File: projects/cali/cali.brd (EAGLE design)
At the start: 100 x 80 mm, 25 parts, among them Q3 IRF540, T1 BC547, T2 BC547, T3 BC547

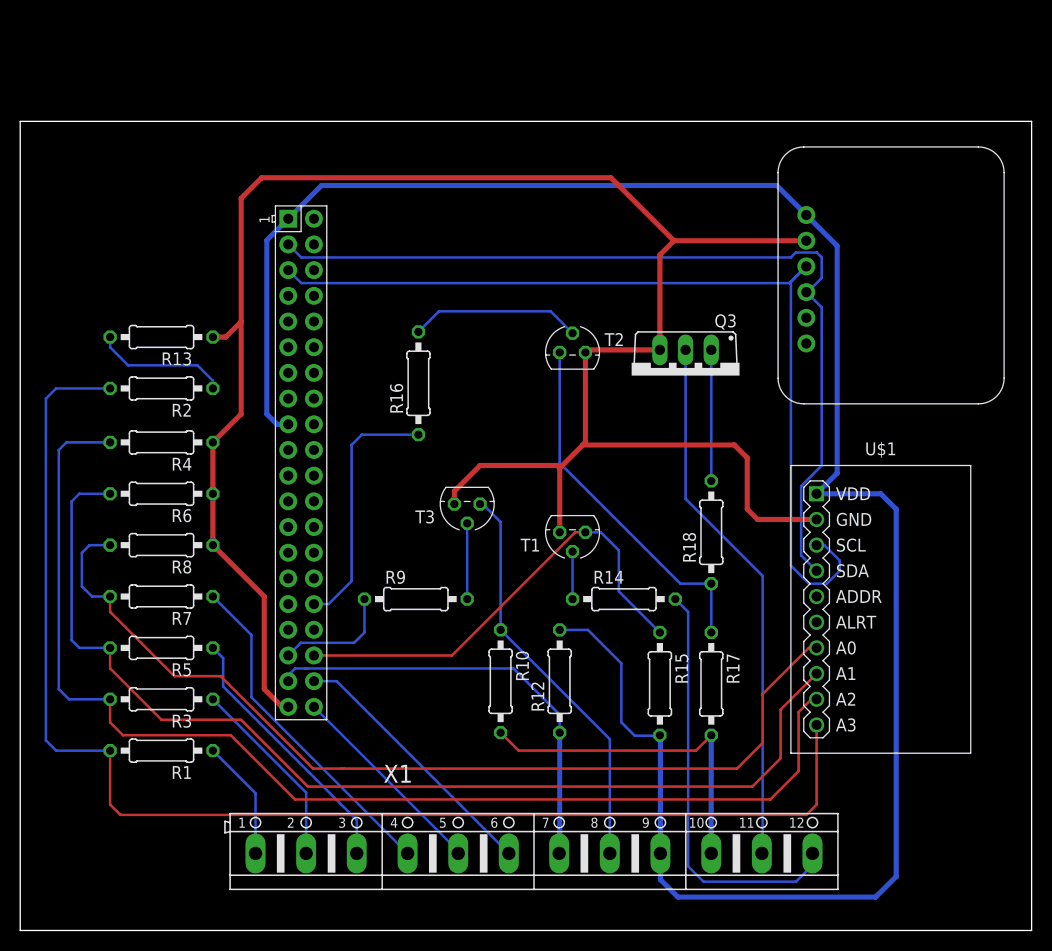
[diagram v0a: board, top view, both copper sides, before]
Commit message: Board v1.0
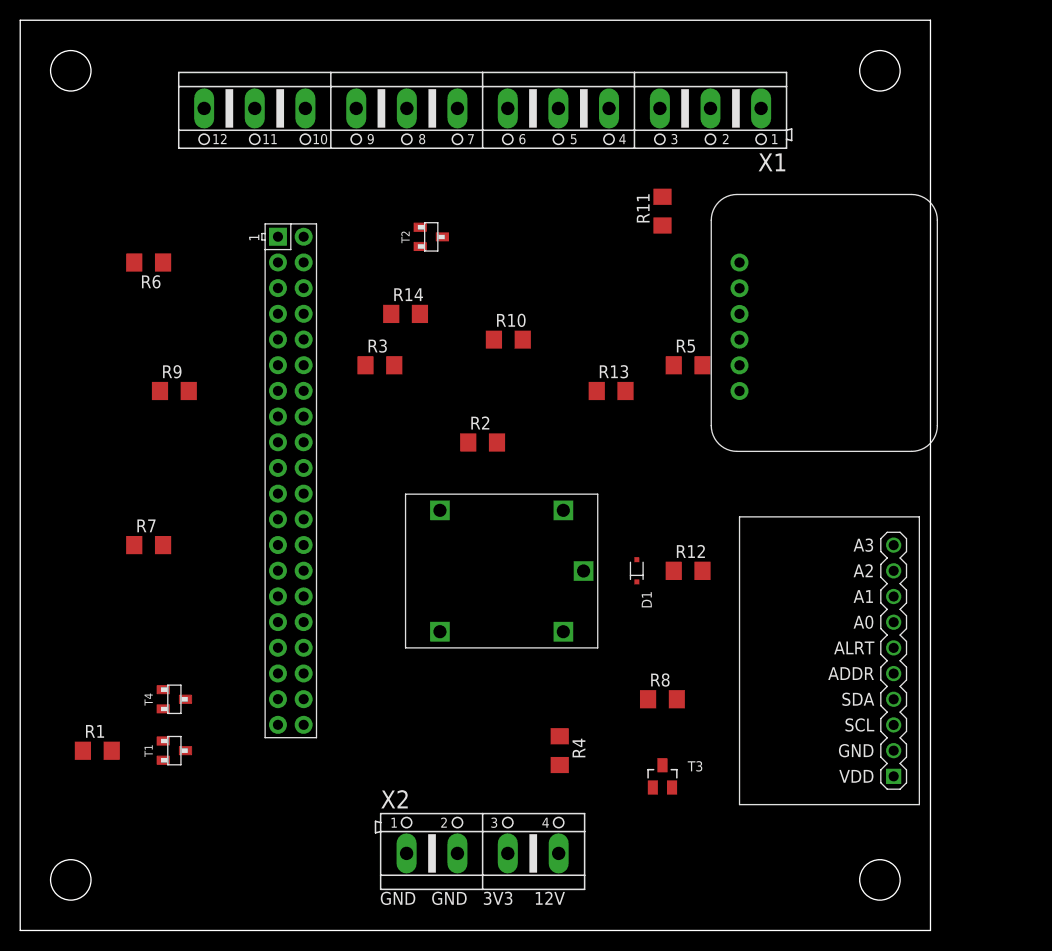
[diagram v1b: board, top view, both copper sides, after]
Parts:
- removed Q3: IRF540, transistor-power:TO220BV
- removed R15, R17: 10k, rcl:0207/10
- removed R16: 1k, rcl:0207/10
- removed R18: 10, rcl:0207/10
- added D1: BAS316, nxp_60:SOD323(F)
- added R11: 10k, rcl:R1206
- added T4: IRLML2502, we-transistor:SOT23
- added U$4: FINDER-36.11, relay2:FINDER-36.11
- added X2: (no value), con-ptr500:AK500/4
- R1: value 0 -> 100; device rcl:0207/10 -> rcl:R1206
- R10: value 10k -> 1k; device rcl:0207/10 -> rcl:R1206
- R12: value 4k7 -> 1k; device rcl:0207/10 -> rcl:R1206
- R13: value 1k -> 0; device rcl:0207/10 -> rcl:R1206
- R14: value 10k -> 2k; device rcl:0207/10 -> rcl:R1206
- R2, R6: value 1k -> 100; device rcl:0207/10 -> rcl:R1206
- R3, R4, R5, R7, R8: device rcl:0207/10 -> rcl:R1206
- R9: value 1k -> 10k; device rcl:0207/10 -> rcl:R1206
- T1, T2: value BC547 -> IRLML2502; device transistor:TO92 -> we-transistor:SOT23
- T3: value BC547 -> 2N7002E; device transistor:TO92 -> nxp_60:SOT23
- moved X1 73.8 mm to (45.7, 81.3), turned to 180 degrees
- moved R5 59.1 mm to (66.0, 55.9), turned to 0 degrees
- moved R8 51.8 mm to (63.5, 22.9), turned to 0 degrees
- moved R4 49.8 mm to (53.3, 17.8), turned to 270 degrees
- moved T1 44.9 mm to (15.2, 17.8), turned to 0 degrees
- moved R13 44.8 mm to (58.4, 53.3), turned to 0 degrees
- moved R3 39.5 mm to (35.6, 55.9), turned to 0 degrees
- moved R14 35.5 mm to (38.1, 61.0)
- moved R10 33.8 mm to (48.3, 58.4), turned to 0 degrees
- moved T3 33.1 mm to (63.5, 15.2), turned to 0 degrees
- moved R2 32.2 mm to (45.7, 48.3), turned to 0 degrees
- moved R9 31.5 mm to (15.2, 53.3)
- moved R6 22.9 mm to (12.7, 66.0)
- moved T2 18.1 mm to (40.6, 68.6)
- moved R12 16.8 mm to (66.0, 35.6), turned to 0 degrees
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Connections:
- removed net 5V0@1: U$2.2
- removed net N$16: Q3.G, R18.2
- removed net N$17: Q3.D, X1.11
- removed net N$18: R12.1, U$2.37, X1.7
- removed net N$20: U$2.40, X1.5
- removed net N$21: U$2.38, X1.6
- removed net N$22: R9.2, T3.2
- removed net N$23: R10.1, T3.3, X1.8
- new net ADC0: U$1.7
- new net ADC1: R7.1, R8.1, U$1.8
- new net ADC2: R10.1, R9.1, U$1.9
- new net ADC3: R11.1, R12.1, U$1.10
- new net ADC4: R13.1, R14.1
- new net GPIO12: R6.1, U$2.32
- new net GPIO16: R1.1, U$2.36
- new net GPIO20: T2.2, U$2.38
- new net GPIO21: R5.1, T3.3, U$2.40
- new net GPIO26: U$2.37, X1.5
- net +12V: now also D1.1, R3.2, R4.2, U$4.A1, X2.4; no longer R10.2, R17.2, X1.10
- net +3V3: now also R2.2, R5.2, X2.3; no longer R12.2, R15.2, X1.9
- net GND: now also R10.2, R12.2, R14.2, R8.2, T1.2, T4.2, U$2.6, X2.1, X2.2; no longer Q3.S, R13.1, R4.1, R6.1, R8.1, T1.1, T2.1, T3.1
- net GPIO19: no longer R9.1
- net N$1: now also D1.2, T4.3, U$4.A2; no longer R1.1, X1.1
- net N$10: now also R2.1, T2.1; no longer R14.1, T1.2
- net N$11: now also R3.1, T2.3, X1.10; no longer R14.2, X1.12
- net N$12: now also R4.1, T3.1; no longer R15.1, T1.3, U$2.36
- net N$13: now also T3.2, X1.9; no longer R16.2, T2.2
- net N$14: now also R11.2, X1.3; no longer R16.1, U$2.32
- net N$15: now also R13.2, X1.4; no longer R17.1, R18.1, T2.3
- net N$2: now also T1.3, X1.11; no longer R3.1, X1.2
- net N$3: now also U$4.NO, X1.8; no longer R5.1, X1.3
- net N$4: now also R6.2, T4.1; no longer R7.1, X1.4
- net N$5: now also U$4.COM, X1.6; no longer R1.2, R2.2, U$1.10
- net N$6: now also R1.2, T1.1; no longer R3.2, R4.2, U$1.9
- net N$7: now also U$4.NC, X1.7; no longer R13.2, R2.1
- net N$8: now also X1.1; no longer R8.2, U$1.7
- net N$9: now also R9.2, X1.2; no longer R5.2, R6.2, U$1.8
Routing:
- net +3V3: track 207.9 -> 0.00 mm
- net GND: track 197.3 -> 0.00 mm
- net N$5: track 131.2 -> 0.00 mm
- net N$6: track 117.3 -> 0.00 mm
- net N$9: track 106.1 -> 0.00 mm
- net N$8: track 95.4 -> 0.00 mm
- net SCL: track 92.7 -> 0.00 mm
- net SDA: track 87.5 -> 0.00 mm
- net N$17: track 53.0 -> 0.00 mm
- net N$12: track 45.7 -> 0.00 mm
- net N$18: track 43.6 -> 0.00 mm
- net N$11: track 41.8 -> 0.00 mm
- net N$23: track 40.0 -> 0.00 mm
- net N$15: track 35.7 -> 0.00 mm
- net +12V: track 33.9 -> 0.00 mm
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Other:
- board size 100 x 80 mm -> 90 x 90 mm
- board text added: "12V"
- board text added: "3V3"
- board text added: "GND"

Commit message: Caliboard 1.0 routing done
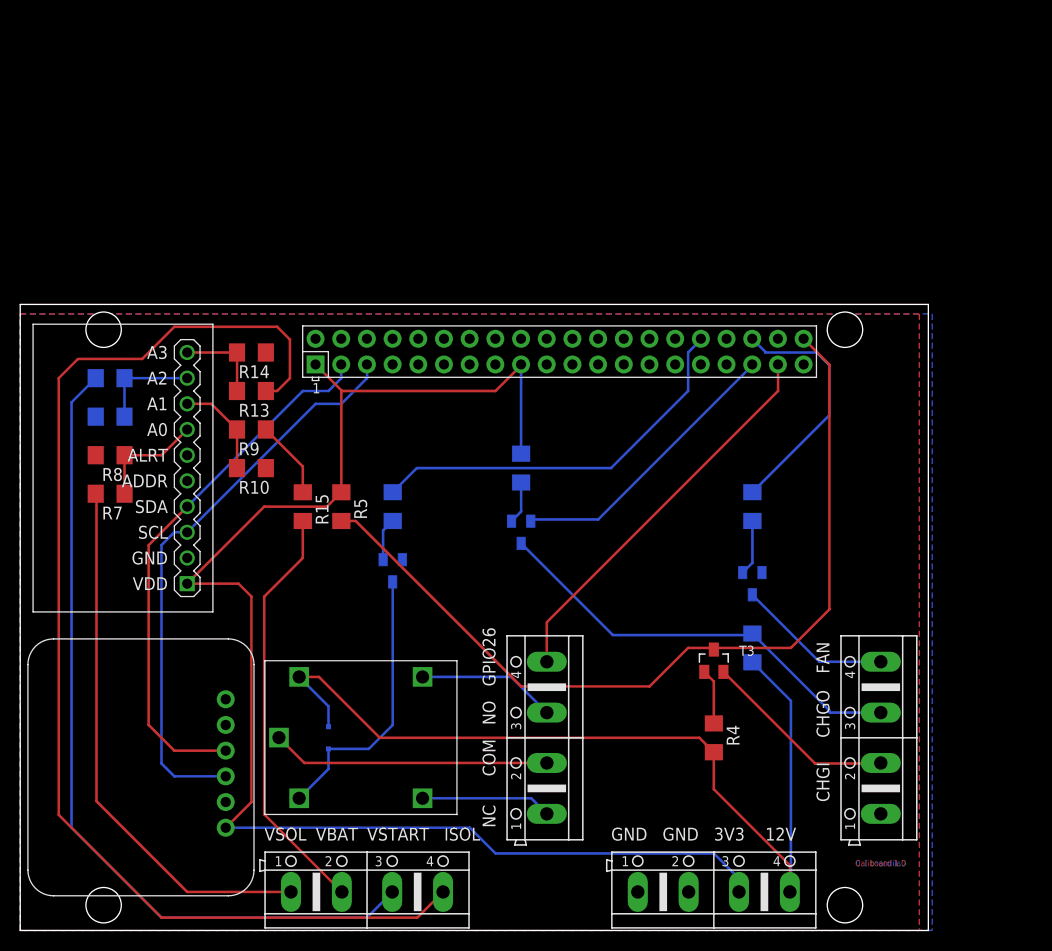
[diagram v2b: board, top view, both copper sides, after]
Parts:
- added R15: 0, rcl:R1206
- added X3, X4: (no value), con-ptr500:AK500/4
- X1: device con-ptr500:AK500/12 -> con-ptr500:AK500/4
- moved U$3 82.8 mm to (23.1, 3.43), turned to 90 degrees
- moved X1 73.6 mm to (85.1, 19.1), turned to 90 degrees
- moved U$1 72.4 mm to (10.2, 45.7)
- moved R1 69.1 mm to (72.4, 41.9), flipped to the bottom, turned to 270 degrees
- moved R8 59.7 mm to (8.89, 47.0), turned to 180 degrees
- moved T1 59.5 mm to (72.4, 34.3), flipped to the bottom, turned to 270 degrees
- moved R12 59.1 mm to (8.89, 50.8), flipped to the bottom
- moved R11 57.1 mm to (8.89, 54.6), flipped to the bottom, turned to 0 degrees
- moved U$2 50.6 mm to (20.8, 30.7), turned to 0 degrees
- moved R3 46.2 mm to (72.4, 27.9), flipped to the bottom, turned to 270 degrees
- moved R5 37.0 mm to (31.8, 41.9), turned to 90 degrees
- moved R13 35.6 mm to (22.9, 53.3)
- moved D1 34.7 mm to (30.5, 19.1), flipped to the bottom, turned to 90 degrees
- moved R6 34.1 mm to (36.8, 41.9), flipped to the bottom, turned to 270 degrees
- moved T2 30.5 mm to (49.5, 39.4), flipped to the bottom, turned to 270 degrees
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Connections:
- removed net ADC4: R13.1, R14.1
- removed net N$14: R11.2, X1.3
- removed net N$15: R13.2, X1.4
- new net I_SOL: R13.2, X3.4
- new net V_SOL: R7.2, X3.1
- new net V_START: R11.2, X3.3
- net ADC0: now also R7.1, R8.1
- net ADC1: now also R10.1, R9.1; no longer R7.1, R8.1
- net ADC2: now also R11.1, R12.1; no longer R10.1, R9.1
- net ADC3: now also R13.1, R14.1; no longer R11.1, R12.1
- net GPIO19: now also T2.2
- net GPIO20: no longer T2.2
- net GPIO26: now also X4.4; no longer X1.5
- net N$11: now also X1.3; no longer X1.10
- net N$13: now also R15.1, R9.2; no longer T3.2, X1.9
- net N$2: now also X1.4; no longer X1.11
- net N$3: now also X4.3; no longer X1.8
- net N$5: now also X4.2; no longer X1.6
- net N$7: now also X4.1; no longer X1.7
- net N$8: now also T3.2, X1.2; no longer R7.2, X1.1
- net N$9: now also R15.2, X3.2; no longer R9.2, X1.2
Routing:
- net +3V3: track 0.00 -> 145.4 mm
- net I_SOL: track 0.00 -> 118.8 mm
- net +12V: track 0.00 -> 91.6 mm
- net GPIO21: track 0.00 -> 86.5 mm
- net V_START: track 0.00 -> 82.0 mm
- net SCL: track 0.00 -> 57.0 mm
- net SDA: track 0.00 -> 53.7 mm
- net V_SOL: track 0.00 -> 53.5 mm
- net N$11: track 0.00 -> 42.7 mm
- net N$9: track 0.00 -> 41.4 mm
- net GPIO12: track 0.00 -> 39.1 mm
- net GPIO26: track 0.00 -> 38.9 mm
- net GPIO19: track 0.00 -> 28.4 mm
- net N$1: track 0.00 -> 27.6 mm
- net N$5: track 0.00 -> 27.5 mm
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- added copper zone on layer 1, net GND
- added copper zone on layer 16, net GND
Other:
- board size 90 x 90 mm -> 89.8 x 61.9 mm
- board text added: "CHGI"
- board text added: "CHGO"
- board text added: "COM"
- board text added: "Caliboard 1.0"
- board text added: "FAN"
- board text added: "GPIO26"
- board text added: "ISOL"
- board text added: "NC"
- board text added: "NO"
- board text added: "VBAT"
- board text added: "VSOL"
- board text added: "VSTART"
